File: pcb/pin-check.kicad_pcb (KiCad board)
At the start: 2 copper layers, 76.2 x 52.3 mm, 55 parts, among them J1 AVR-ISP-6, J2 SJ-43514, P1 USB_C_Receptacle_USB2.0, SW1 MX-NoLED, SW2 MX-NoLED, SW3 MX-NoLED, SW4 MX-NoLED, SW7 Reset, SW8 Boot, U1 ATmega328P-PU, Y1 16MHz

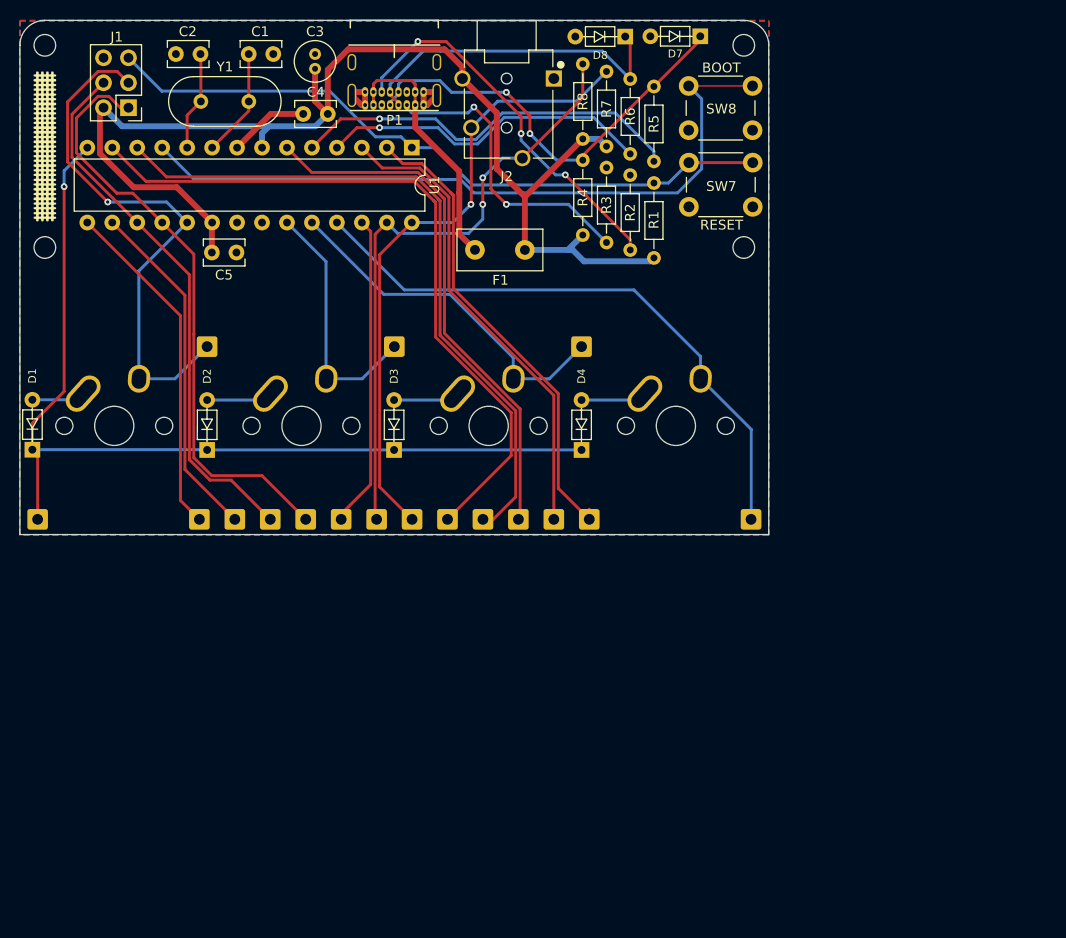
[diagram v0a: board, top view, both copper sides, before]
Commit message: some changes
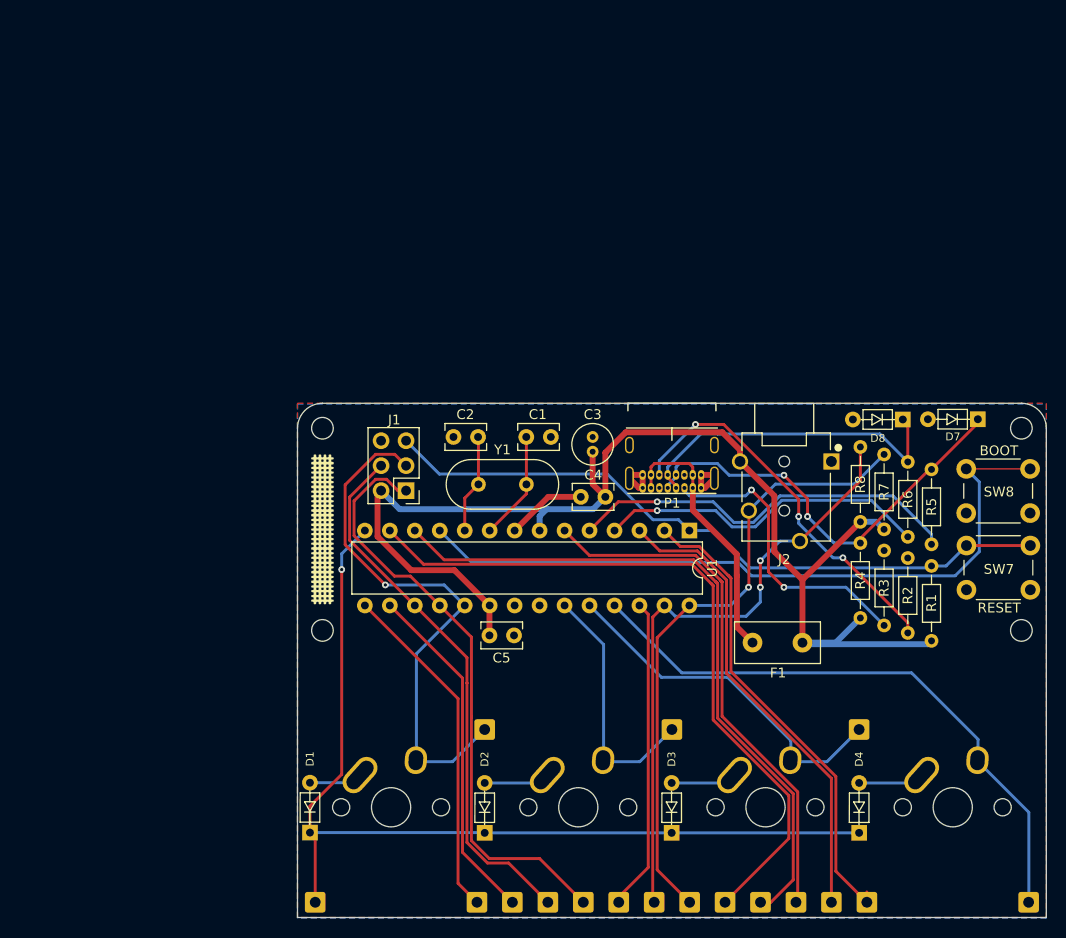
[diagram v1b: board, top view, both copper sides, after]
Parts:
- moved F1 48.9 mm to (162.2, 88.7)
- moved H7 48.1 mm to (165.1, 115.1)
- moved D1 48.1 mm to (112.1, 109.3)
- moved D3 48.1 mm to (148.9, 109.3)
- moved G*** 48.1 mm to (113.3, 77.2)
- moved H1 48.1 mm to (112.6, 115.1)
- moved H10 48.1 mm to (154.3, 115.1)
- moved H11 48.1 mm to (150.7, 115.1)
- moved H14 48.1 mm to (139.9, 115.1)
- moved H2 48.1 mm to (129.8, 97.6)
- moved H3 48.1 mm to (148.9, 97.6)
- moved H4 48.1 mm to (167.9, 97.6)
- moved J1 48.1 mm to (121.8, 73.3)
- moved P1 48.1 mm to (148.9, 66.9)
- moved R5 48.1 mm to (175.3, 78.7)
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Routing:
- net +5V: track 121.9 -> 127.3 mm
- net Net-(F1-Pad2): track 26.1 -> 27.1 mm
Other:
- board text added: "ColA"
- board text added: "ColB"
- board text added: "ColC"
- board text added: "ColD"
- board text added: "SW1"
- board text added: "SW2"
- board text added: "SW3"
- board text added: "SW4"
